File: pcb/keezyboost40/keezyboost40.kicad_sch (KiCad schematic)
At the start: 89 parts, among them SW1 SW_SPST, SW10 SW_SPST, SW11 SW_SPST, SW12 SW_SPST, SW13 SW_SPST, SW14 SW_SPST, SW15 SW_SPST, SW16 SW_SPST, SW17 SW_SPST, SW18 SW_SPST, SW19 SW_SPST, SW2 SW_SPST, SW20 SW_SPST, SW21 SW_SPST, SW22 SW_SPST, SW23 SW_SPST, SW24 SW_SPST, SW25 SW_SPST, SW26 SW_SPST, SW27 SW_SPST, SW28 SW_SPST, SW29 SW_SPST, SW3 SW_SPST, SW30 SW_SPST, SW31 SW_SPST, SW32 SW_SPST, SW33 SW_SPST, SW34 SW_SPST, SW35 SW_SPST, SW36 SW_SPST, SW37 SW_SPST, SW38 SW_SPST, SW39 SW_SPST, SW4 SW_SPST, SW40 SW_SPST, SW5 SW_SPST, SW6 SW_SPST, SW7 SW_SPST, SW8 SW_SPST, SW9 SW_SPST, U1 Pico, U2 ST7735_1.8inch

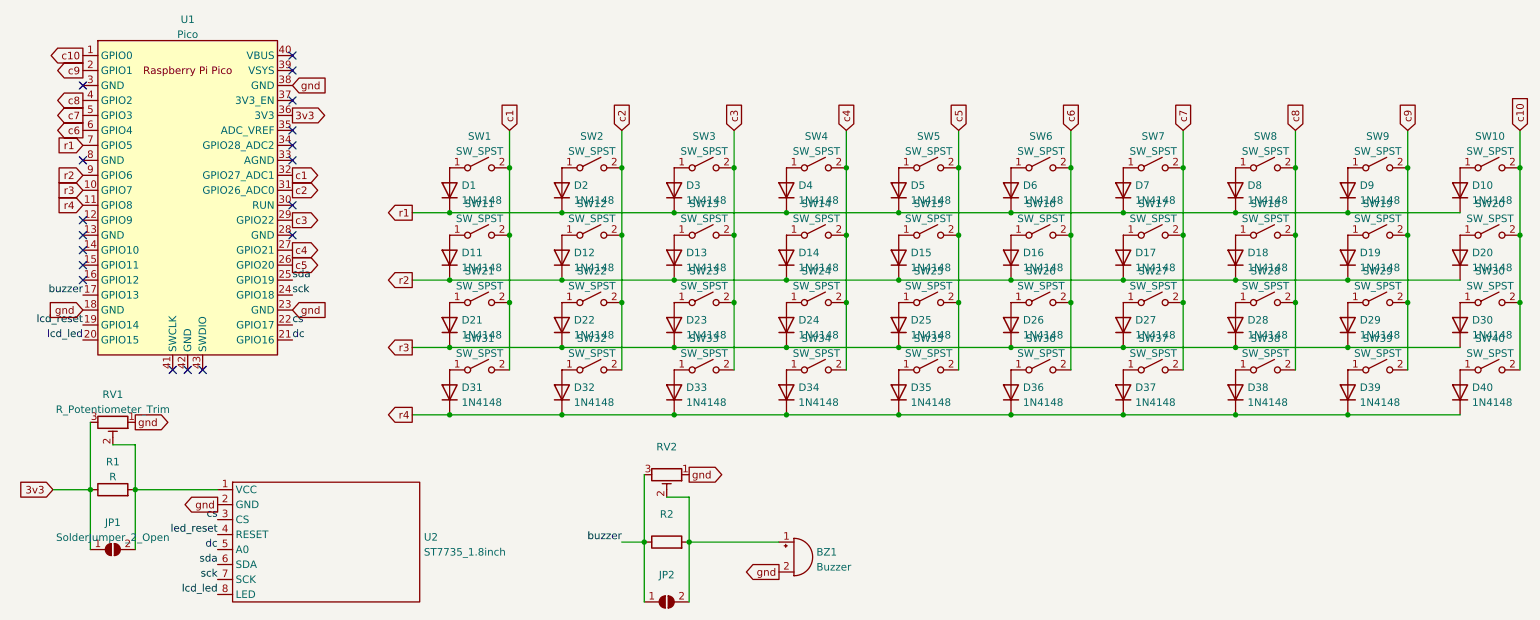
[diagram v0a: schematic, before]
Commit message: finish v0.0
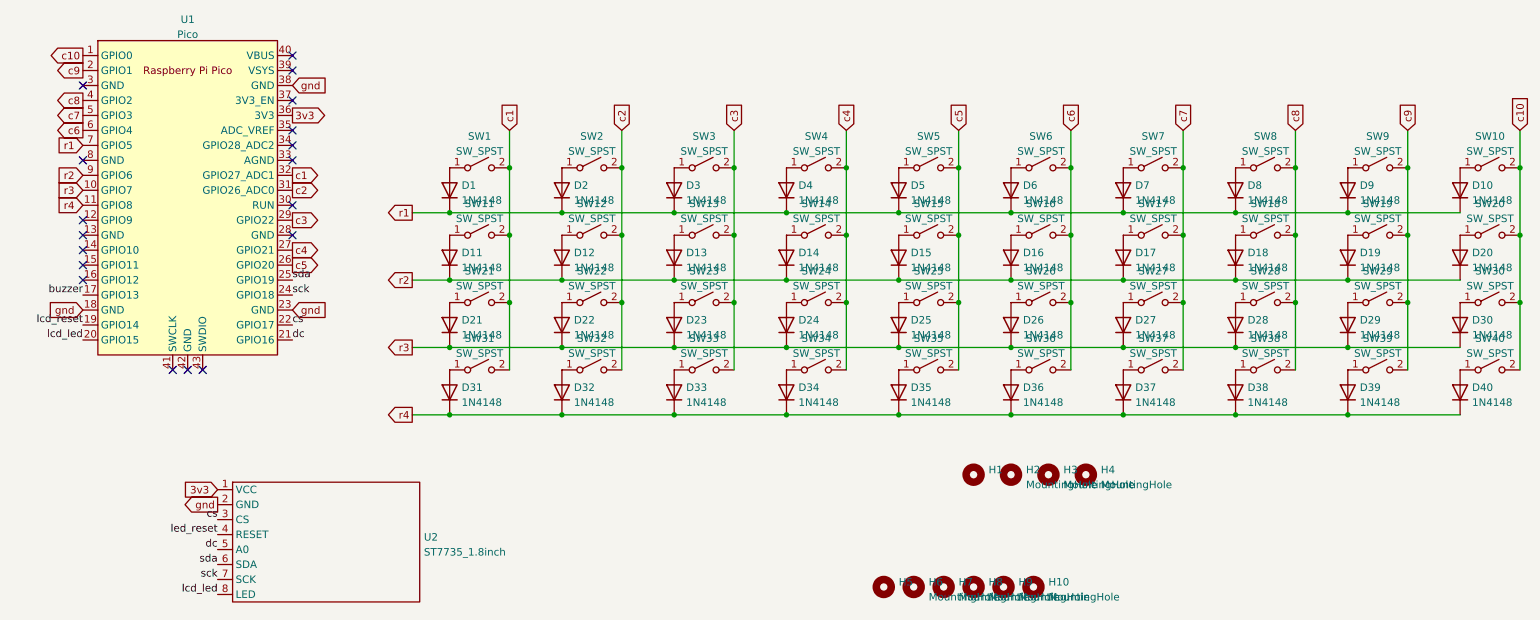
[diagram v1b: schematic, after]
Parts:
- removed BZ1: Buzzer, symbol Device:Buzzer
- removed JP1: SolderJumper_2_Open, symbol Jumper:SolderJumper_2_Open
- removed JP2: (no value), symbol Jumper:SolderJumper_2_Open
- removed R1: R, symbol Device:R
- removed R2: (no value), symbol Device:R
- removed RV1: R_Potentiometer_Trim, symbol Device:R_Potentiometer_Trim
- removed RV2: (no value), symbol Device:R_Potentiometer_Trim
- added H1, H5: (no value), symbol Mechanical:MountingHole
- added H10, H2, H3, H4, H6, H7, H8, H9: MountingHole, symbol Mechanical:MountingHole
- U1: footprint RPi_Pico:RPi_Pico_SMD_TH -> (none)
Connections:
- net 3v3: now also U2.1 (VCC)
